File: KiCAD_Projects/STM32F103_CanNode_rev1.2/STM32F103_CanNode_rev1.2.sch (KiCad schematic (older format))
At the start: 77 parts, among them P1 CONN_01X04, P10 CONN_01X04, P11 CONN_01X04, P12 CONN_01X02, P2 CONN_01X04, P3 CONN_01X08, P4 CONN_01X08, P5 CONN_01X06, P6 CONN_01X02, P7 CONN_01X08, P8 CONN_01X04, P9 CONN_01X04, SW1 SW_PUSH, SW2 SW_PUSH, U1 STM32F103_48, U2 AOZ1280, U3 MAX3051, U4 NCP1117ST50T3G, U5 TBD62083A, X2 CRYSTAL

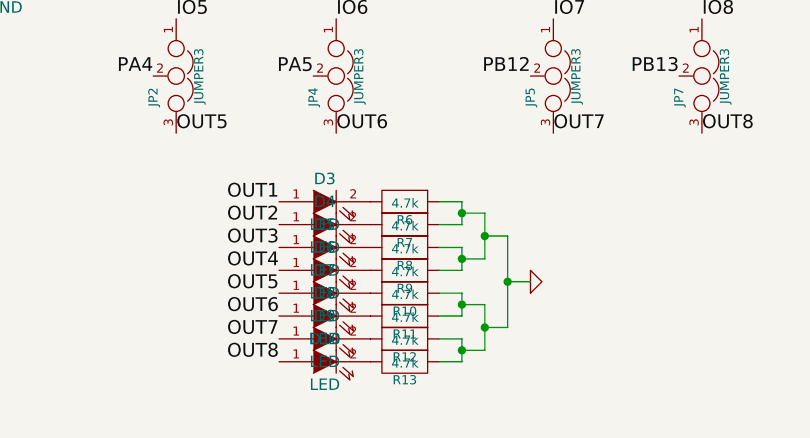
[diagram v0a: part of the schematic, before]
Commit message: セルチェッカー作った｡電源基板ver1.1作った｡ぶっさしMDいじった｡DCDCいじりだした｡
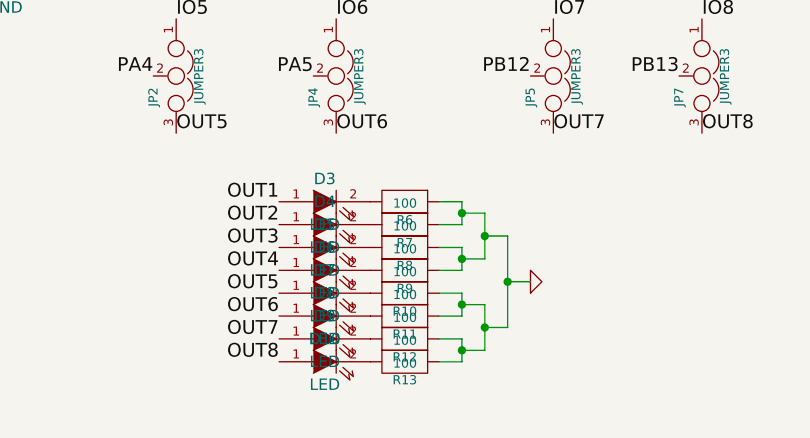
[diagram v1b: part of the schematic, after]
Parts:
- R10, R11, R12, R13, R6, R7, R8, R9: value 4.7k -> 100
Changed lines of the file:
@@
 P 6500 8100
 F 0 "R6" V 6580 8100 40  0000 C CNN
-F 1 "4.7k" V 6507 8101 40  0000 C CNN
+F 1 "100" V 6507 8101 40  0000 C CNN
 F 2 "RP_KiCAD_Libs:C1608_WP" V 6430 8100 30  0001 C CNN
 F 3 "" H 6500 8100 30  0000 C CNN
@@
 P 6500 8200
 F 0 "R7" V 6580 8200 40  0000 C CNN
-F 1 "4.7k" V 6507 8201 40  0000 C CNN
+F 1 "100" V 6507 8201 40  0000 C CNN
 F 2 "RP_KiCAD_Libs:C1608_WP" V 6430 8200 30  0001 C CNN
 F 3 "" H 6500 8200 30  0000 C CNN
@@
 P 6500 8300
 F 0 "R8" V 6580 8300 40  0000 C CNN
-F 1 "4.7k" V 6507 8301 40  0000 C CNN
+F 1 "100" V 6507 8301 40  0000 C CNN
 F 2 "RP_KiCAD_Libs:C1608_WP" V 6430 8300 30  0001 C CNN
 F 3 "" H 6500 8300 30  0000 C CNN
@@
 P 6500 8400
 F 0 "R9" V 6580 8400 40  0000 C CNN
-F 1 "4.7k" V 6507 8401 40  0000 C CNN
+F 1 "100" V 6507 8401 40  0000 C CNN
 F 2 "RP_KiCAD_Libs:C1608_WP" V 6430 8400 30  0001 C CNN
 F 3 "" H 6500 8400 30  0000 C CNN
@@
 P 6500 8500
 F 0 "R10" V 6580 8500 40  0000 C CNN
-F 1 "4.7k" V 6507 8501 40  0000 C CNN
+F 1 "100" V 6507 8501 40  0000 C CNN
 F 2 "RP_KiCAD_Libs:C1608_WP" V 6430 8500 30  0001 C CNN
 F 3 "" H 6500 8500 30  0000 C CNN
@@
 P 6500 8600
 F 0 "R11" V 6580 8600 40  0000 C CNN
-F 1 "4.7k" V 6507 8601 40  0000 C CNN
+F 1 "100" V 6507 8601 40  0000 C CNN
 F 2 "RP_KiCAD_Libs:C1608_WP" V 6430 8600 30  0001 C CNN
 F 3 "" H 6500 8600 30  0000 C CNN
@@
 P 6500 8700
 F 0 "R12" V 6580 8700 40  0000 C CNN
-F 1 "4.7k" V 6507 8701 40  0000 C CNN
+F 1 "100" V 6507 8701 40  0000 C CNN
 F 2 "RP_KiCAD_Libs:C1608_WP" V 6430 8700 30  0001 C CNN
 F 3 "" H 6500 8700 30  0000 C CNN
@@
 P 6500 8800
 F 0 "R13" V 6580 8800 40  0000 C CNN
-F 1 "4.7k" V 6507 8801 40  0000 C CNN
+F 1 "100" V 6507 8801 40  0000 C CNN
 F 2 "RP_KiCAD_Libs:C1608_WP" V 6430 8800 30  0001 C CNN
 F 3 "" H 6500 8800 30  0000 C CNN
